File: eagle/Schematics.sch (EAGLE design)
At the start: 56 parts, among them IC1 ADE9000, K1 PIN20X2

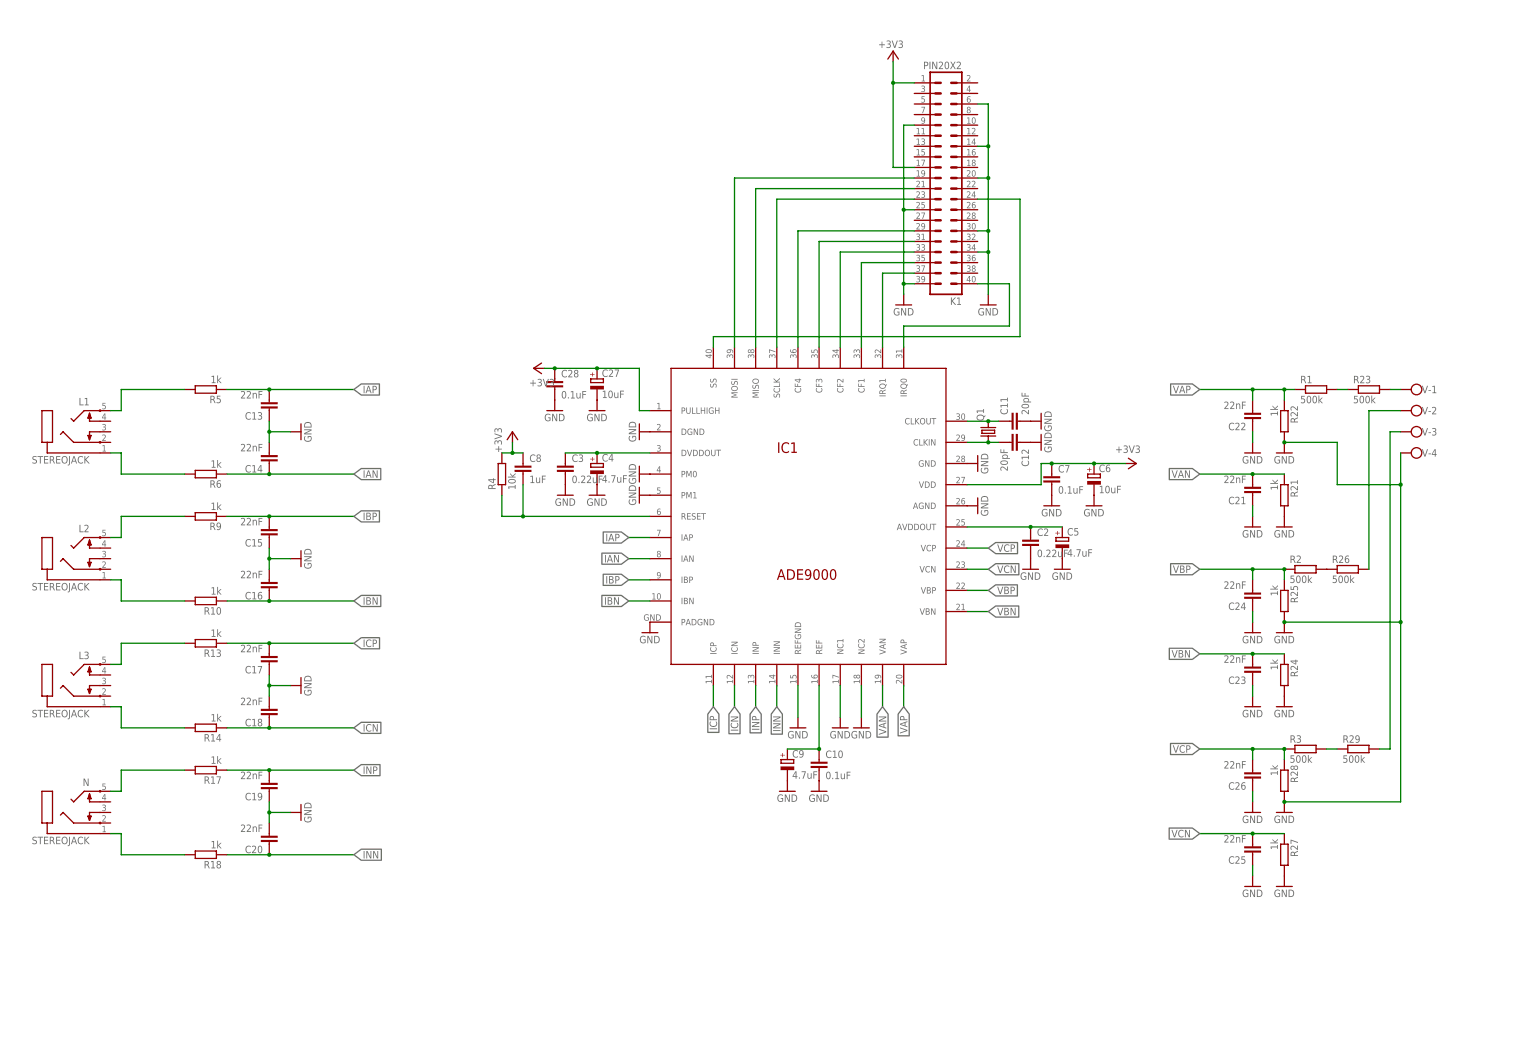
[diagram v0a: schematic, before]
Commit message: Changes
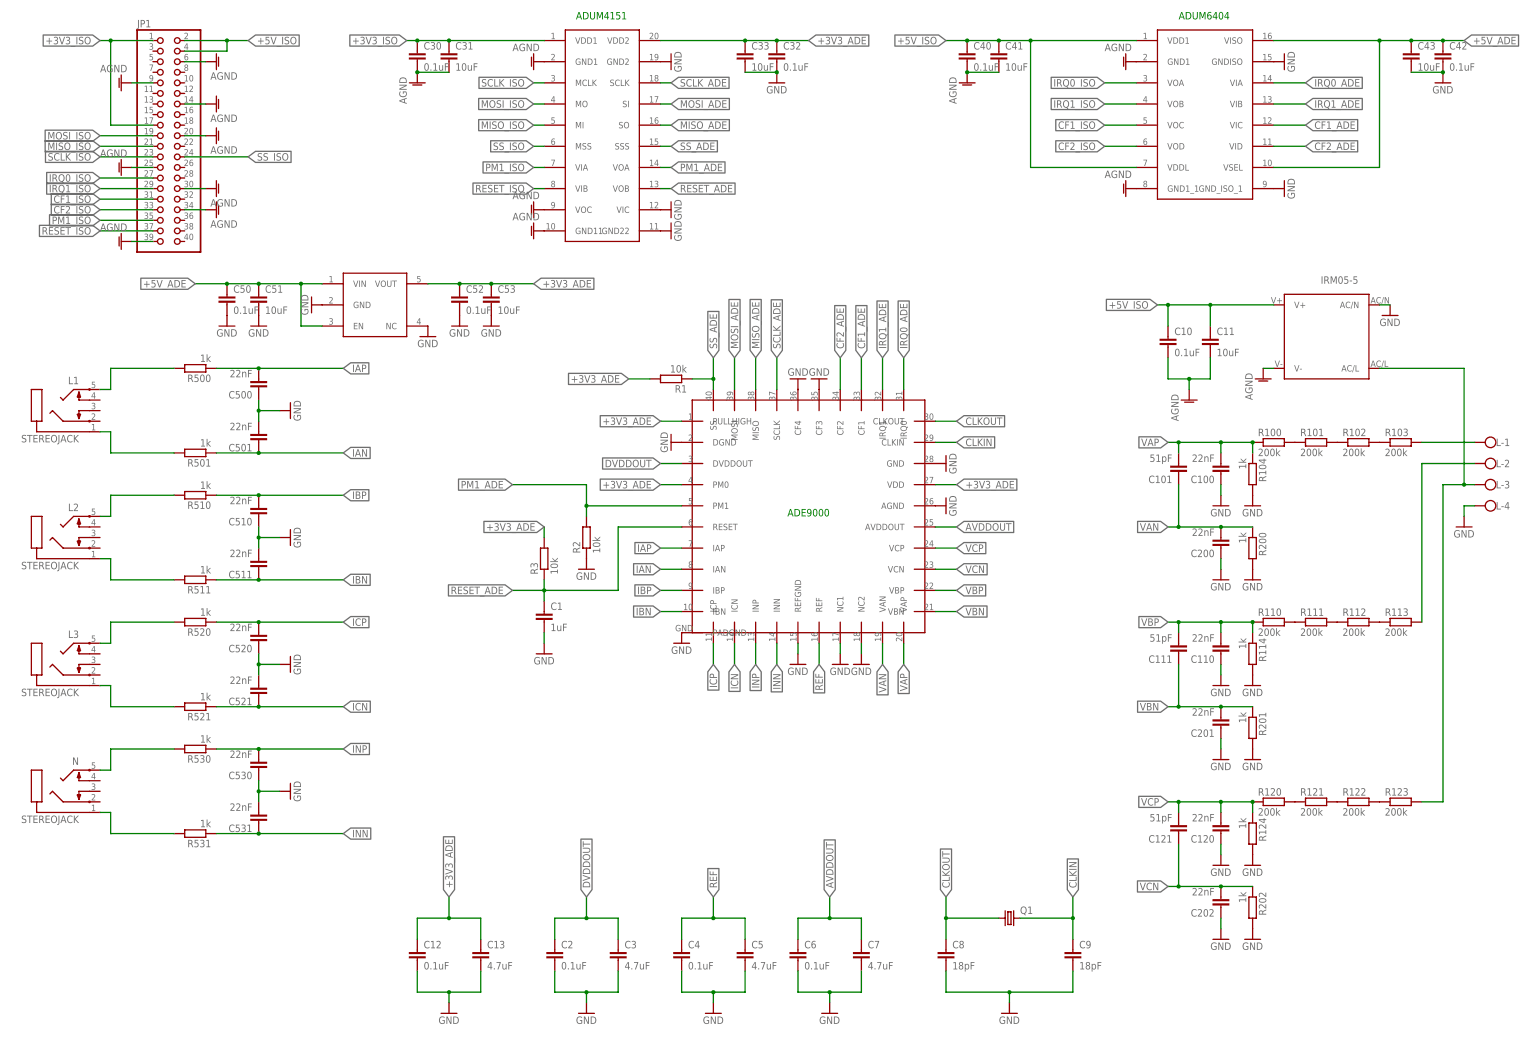
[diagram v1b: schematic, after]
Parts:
- removed C14, C15, C16, C17, C18, C19, C20, C21, C22, C23, C24, C25, C26: 22nF, resistor:C-EUC0805
- removed C27: 10uF, resistor:CPOL-EUC
- removed C28: 0.1uF, resistor:C-EUC0805
- removed IC1: ADE9000, ADE9000:ADE9000
- removed K1: PIN20X2, FLYFISH:PIN20X2
- removed R10, R13, R14, R17, R18, R21, R22, R24, R25, R27, R28, R5, R6, R9: 1k, resistor:R-EU_M0805
- removed R23, R26, R29: 500k, resistor:R-EU_M1206
- removed R4: 10k, resistor:R-EU_M0805
- removed V: (no value), con-wago-500:W237-4
- added ADE9000: ADE9000, ADE9000:ADE9000
- added ADUM4151: ADUM4151, ADUM4151:ADUM4151
- added ADUM6404: ADUM6404, ADUM6404:ADUM6404
- added C1: 1uF, resistor:C-EUC0805
- added C100, C110, C120, C200, C201, C202, C500, C501, C510, C511, C520, C521, C530, C531: 22nF, resistor:C-EUC0805
- added C101, C111, C121: 51pF, resistor:C-EUC0805
- added C30, C32, C40, C42, C50, C52: 0.1uF, resistor:C-EUC0805
- added C31, C33, C41, C43, C51, C53: 10uF, resistor:C-EUC0805
- added IRM05-5: (no value), meanwell_irm_v6:IRM_05/10
- added JP1: (no value), adafruit:PINHD-2X20
- added L: (no value), con-wago-500:W237-4
- added R100, R101, R102, R103, R110, R111, R112, R113, R120, R121, R122, R123: 200k, resistor:R-EU_M1206
- added R104, R114, R124, R200, R201, R202, R500, R501, R510, R511, R520, R521, R530, R531: 1k, resistor:R-EU_M0805
- added U$5: ADP122AUJZ-3.3-R7, ADP122AUJZ-3.3-R7:ADP122AUJZ-3.3-R7
- C11: value 20pF -> 10uF
- C12: value 20pF -> 0.1uF
- C13: value 22nF -> 4.7uF
- C2: value 0.22uF -> 0.1uF
- C3: value 0.22uF -> 4.7uF
- C4: value 4.7uF -> 0.1uF; device resistor:CPOL-EUC -> resistor:C-EUC0805
- C5: device resistor:CPOL-EUC -> resistor:C-EUC0805
- C6: value 10uF -> 0.1uF; device resistor:CPOL-EUC -> resistor:C-EUC0805
- C7: value 0.1uF -> 4.7uF
- C8: value 1uF -> 18pF
- C9: value 4.7uF -> 18pF; device resistor:CPOL-EUC -> resistor:C-EUC0805
- Q1: device crystal:CRYSTALHC49UP -> crystal:CRYSTALCTS406
- R1, R2, R3: value 500k -> 10k; device resistor:R-EU_M1206 -> resistor:R-EU_M0805
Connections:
- removed net +3V3: C27.+, C28.1, C6.+, C7.1, C8.1, IC1.PULLHIGH, IC1.VDD, K1.1, K1.17, R4.2
- removed net N$2: IC1.CF1, K1.35
- removed net N$24: IC1.MOSI, K1.19
- removed net N$25: IC1.MISO, K1.21
- removed net N$26: IC1.SCLK, K1.23
- removed net N$27: IC1.SS, K1.24
- removed net N$5: C3.1, C4.+, IC1.DVDDOUT
- removed net N$6: C8.2, IC1.RESET, R4.1
- removed net N$7: C10.1, C9.+, IC1.REF
- removed net N$8: C11.1, IC1.CLKOUT, Q1.2
- removed net N$9: C12.2, IC1.CLKIN, Q1.1
- new net +3V3_ADE: ADE9000.PM0, ADE9000.PULLHIGH, ADE9000.VDD, ADUM4151.VDD2, C12.1, C13.1, C32.1, C33.1, C52.1, C53.1, R1.2, R3.2, U$5.VOUT
- new net +3V3_ISO: ADUM4151.VDD1, C30.1, C31.1, JP1.1, JP1.17
- new net +5V_ADE: ADUM6404.VISO, ADUM6404.VSEL, C42.1, C43.1, C50.1, C51.1, U$5.EN, U$5.VIN
- new net +5V_ISO: ADUM6404.VDD1, ADUM6404.VDDL, C10.1, C11.1, C40.1, C41.1, IRM05-5.V+, JP1.2, JP1.4
- new net AGND: ADUM4151.GND1, ADUM4151.GND11, ADUM4151.VOC, ADUM6404.GND1, ADUM6404.GND1_1, C10.2, C11.2, C30.2, C31.2, C40.2, C41.2, IRM05-5.V-, JP1.14, JP1.20, JP1.25, JP1.30, JP1.34, JP1.39, JP1.6, JP1.9
- new net AVDDOUT: ADE9000.AVDDOUT, C6.1, C7.1
- new net CF1_ADE: ADE9000.CF1, ADUM6404.VIC
- new net CF1_ISO: ADUM6404.VOC, JP1.31
- new net CF2_ADE: ADE9000.CF2, ADUM6404.VID
- new net CF2_ISO: ADUM6404.VOD, JP1.33
- new net CLKIN: ADE9000.CLKIN, C9.1, Q1.2
- new net CLKOUT: ADE9000.CLKOUT, C8.1, Q1.1
- new net DVDDOUT: ADE9000.DVDDOUT, C2.1, C3.1
- new net IRQ0_ADE: ADE9000.IRQ0, ADUM6404.VIA
- new net IRQ0_ISO: ADUM6404.VOA, JP1.27
- new net IRQ1_ADE: ADE9000.IRQ1, ADUM6404.VIB
- new net IRQ1_ISO: ADUM6404.VOB, JP1.29
- new net MISO_ADE: ADE9000.MISO, ADUM4151.SO
- new net MISO_ISO: ADUM4151.MI, JP1.21
- new net MOSI_ADE: ADE9000.MOSI, ADUM4151.SI
- new net MOSI_ISO: ADUM4151.MO, JP1.19
- new net PM1_ADE: ADE9000.PM1, ADUM4151.VOA, R2.2
- new net PM1_ISO: ADUM4151.VIA, JP1.35
- new net REF: ADE9000.REF, C4.1, C5.1
- new net RESET_ADE: ADE9000.RESET, ADUM4151.VOB, C1.1, R3.1
- new net RESET_ISO: ADUM4151.VIB, JP1.37
- new net SCLK_ADE: ADE9000.SCLK, ADUM4151.SCLK
- new net SCLK_ISO: ADUM4151.MCLK, JP1.23
- new net SS_ADE: ADE9000.SS, ADUM4151.SSS, R1.1
- new net SS_ISO: ADUM4151.MSS, JP1.24
- net GND: now also ADE9000.AGND, ADE9000.CF3, ADE9000.CF4, ADE9000.DGND, ADE9000.GND, ADE9000.NC1, ADE9000.NC2, ADE9000.PADGND, ADE9000.REFGND, ADUM4151.GND2, ADUM4151.GND22, ADUM4151.VIC, ADUM6404.GNDISO, ADUM6404.GND_ISO_1, C1.2, C100.1, C110.1, C12.2, C120.1, C13.2, C200.1, C201.1, C202.1, C32.2, C33.2, C4.2, C42.2, C43.2, C5.2, C50.2, C500.1, C501.2, C51.2, C510.1, C511.2, C52.2, C520.1, C521.2, C53.2, C530.1, C531.2, C6.2, C8.2, C9.2, IRM05-5.AC/N, L-4.KL, R104.2, R114.2, R124.2, R2.1, R200.2, R201.2, R202.2, U$5.GND, U$5.NC; no longer C10.2, C11.2, C12.1, C13.1, C14.2, C15.1, C16.2, C17.1, C18.2, C19.1, C20.2, C21.1, C22.1, C23.1, C24.1, C25.1, C26.1, C27.-, C28.2, C4.-, C5.-, C6.-, C9.-, IC1.AGND, IC1.DGND, IC1.GND, IC1.NC1, IC1.NC2, IC1.PADGND, IC1.PM0, IC1.PM1, IC1.REFGND, K1.14, K1.20, K1.25, K1.30, K1.34, K1.39, K1.6, K1.9, R21.2, R22.2, R24.2, R25.2, R27.2, R28.2, V-4.KL
- net IAN: now also ADE9000.IAN, C501.1, R501.1; no longer C14.1, IC1.IAN, R6.1
- net IAP: now also ADE9000.IAP, C500.2, R500.1; no longer C13.2, IC1.IAP, R5.1
- net IBN: now also ADE9000.IBN, C511.1, R511.1; no longer C16.1, IC1.IBN, R10.1
- net IBP: now also ADE9000.IBP, C510.2, R510.1; no longer C15.2, IC1.IBP, R9.1
- net ICN: now also ADE9000.ICN, C521.1, R521.1; no longer C18.1, IC1.ICN, R14.1
- net ICP: now also ADE9000.ICP, C520.2, R520.1; no longer C17.2, IC1.ICP, R13.1
- net INN: now also ADE9000.INN, C531.1, R531.1; no longer C20.1, IC1.INN, R18.1
- net INP: now also ADE9000.INP, C530.2, R530.1; no longer C19.2, IC1.INP, R17.1
- net N$1: now also R121.2, R122.1; no longer IC1.IRQ1, K1.37
- net N$10: now also R500.2; no longer R5.2
- net N$11: now also R501.2; no longer R6.2
- net N$12: now also R510.2; no longer R9.2
- net N$13: now also R511.2; no longer R10.2
- net N$14: now also R520.2; no longer R13.2
- net N$15: now also R521.2; no longer R14.2
- net N$16: now also R530.2; no longer R17.2
- net N$17: now also R531.2; no longer R18.2
- net N$18: now also R101.2, R102.1; no longer R23.2, V-1.KL
- net N$19: now also R111.2, R112.1; no longer R26.2, V-2.KL
- net N$20: now also R112.2, R113.1; no longer R29.2, V-3.KL
- net N$21: now also R122.2, R123.1; no longer IC1.CF3, K1.31
- net N$22: now also L-2.KL, R113.2; no longer IC1.CF4, K1.29
- net N$23: now also IRM05-5.AC/L, L-3.KL, R123.2; no longer IC1.IRQ0, K1.40
- net N$29: now also R110.2, R111.1; no longer R2.2, R26.1
- net N$3: now also R102.2, R103.1; no longer IC1.CF2, K1.33
- net N$30: now also R100.2, R101.1; no longer R1.2, R23.1
- net N$31: now also R120.2, R121.1; no longer R29.1, R3.2
- net N$4: now also L-1.KL, R103.2; no longer C2.1, C5.+, IC1.AVDDOUT
- net VAN: now also ADE9000.VAN, C101.1, C200.2, R200.1; no longer C21.2, IC1.VAN, R21.1
- net VAP: now also ADE9000.VAP, C100.2, C101.2, R100.1, R104.1; no longer C22.2, IC1.VAP, R1.1, R22.1
- net VBN: now also ADE9000.VBN, C111.1, C201.2, R201.1; no longer C23.2, IC1.VBN, R24.1
- net VBP: now also ADE9000.VBP, C110.2, C111.2, R110.1, R114.1; no longer C24.2, IC1.VBP, R2.1, R25.1
- net VCN: now also ADE9000.VCN, C121.1, C202.2, R202.1; no longer C25.2, IC1.VCN, R27.1
- net VCP: now also ADE9000.VCP, C120.2, C121.2, R120.1, R124.1; no longer C26.2, IC1.VCP, R28.1, R3.1
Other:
- note added: "ADE9000"
- note added: "ADUM4151"
- note added: "ADUM6404"
- moved on the sheet: C10, C11, C12, C13, C2, C3, C7, C8, L1, L2, L3, N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
